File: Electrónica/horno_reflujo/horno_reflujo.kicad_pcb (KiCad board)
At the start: 2 copper layers, 100 x 80 mm, 46 parts, among them J1 LevelShifter, J10 ssr1, J11 ssr2, J12 encoder, J13 Max6675_modulo2, J14 Max6675_modulo3, J15 Max6675_modulo4, J2 LevelShifter, J3 Display Oled I2C, J4 Max6675_modulo, J5 ESP01, J6 Alimentación y zc, J7 Relevador a ventilador, J8 resistencia, K1 SANYOU_SRD_Form_C, Q1 2N2222A-TO92, U1 LD1117S33TR_SOT223, U2 74LS14

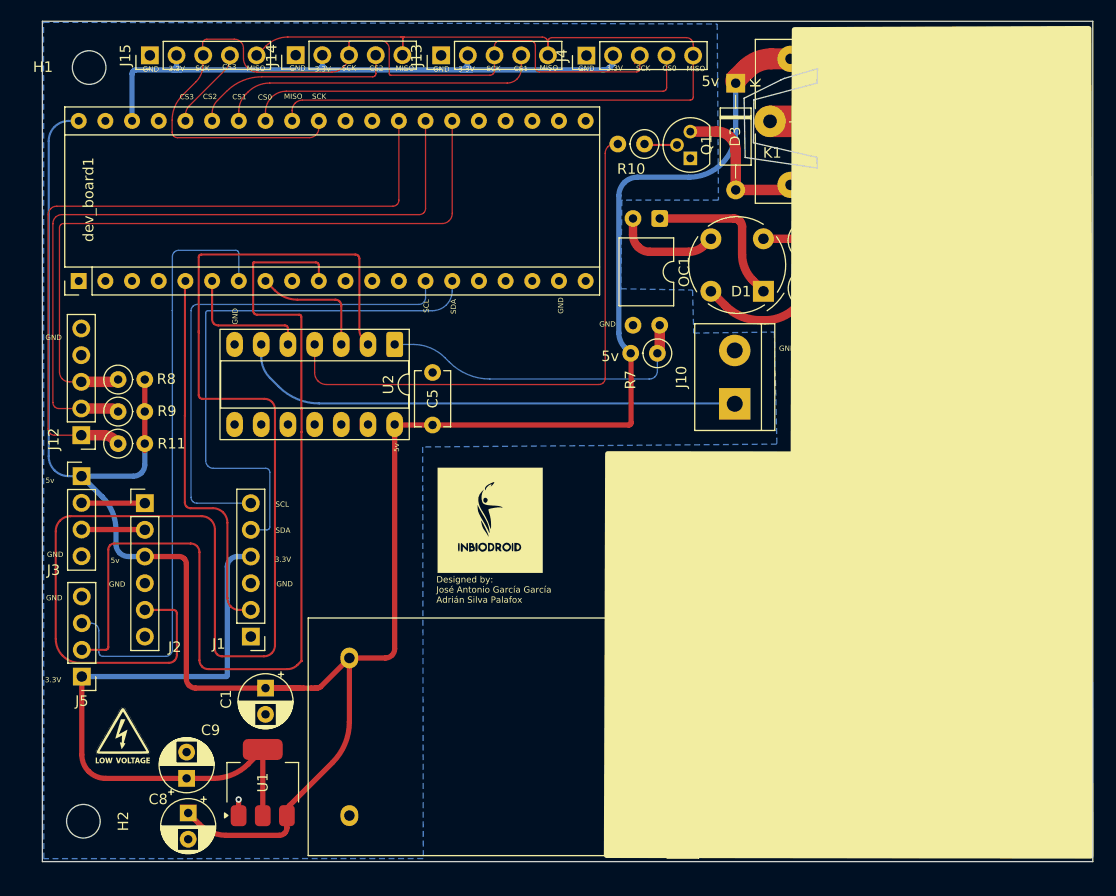
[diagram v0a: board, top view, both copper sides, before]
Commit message: mounting holes update
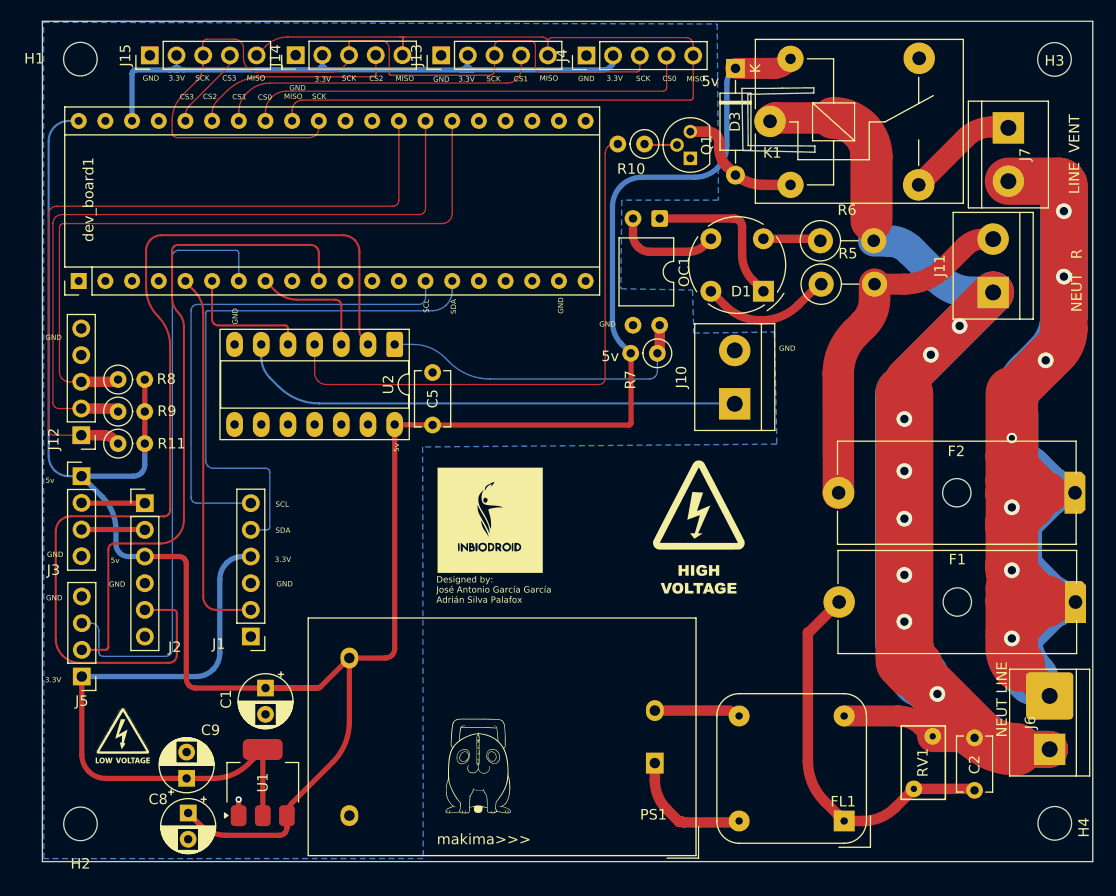
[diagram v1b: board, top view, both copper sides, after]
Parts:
- removed J8: resistencia, Connector_PinHeader_2.54mm:PinHeader_1x01_P2.54mm_Vertical
- added G***: LOGO, LOGO, F.Cu at (76.5, 97.2)
- moved D3 1.41 mm to (101.0, 30.8)
- moved R5 1.28 mm to (109.1, 51.3)
- moved H1 1.16 mm to (38.6, 29.9)
- moved R6 1.15 mm to (109.1, 47.2)
- moved H3 0.55 mm to (131.3, 29.9)
- moved H2 0.37 mm to (38.6, 102.7), turned to 180 degrees
- moved H4 0.20 mm to (131.4, 102.7)
- moved J11 0.11 mm to (125.5, 52.1)
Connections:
- F2 pad 2: Net-(J8-Pin_1) -> Net-(J11-Pin_2)
- J11 pad 2: unconnected-(J11-Pin_2-Pad2) -> Net-(J11-Pin_2)
- R5 pad 2: Net-(J8-Pin_1) -> Net-(J11-Pin_2)
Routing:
- net zero: track 133.3 -> 99.1 mm
- net Net-(J11-Pin_2): track 0.00 -> 33.6 mm
- net /Rx_mcu_esp01: track 92.3 -> 64.0 mm
- net Net-(J8-Pin_1): track 27.5 -> 0.00 mm
- net NEUT: track 176.7 -> 172.0 mm
- net Net-(D1-1): track 4.32 -> 6.62 mm
- net +3.3Vmc: track 58.5 -> 60.7 mm
- net +5V: track 224.9 -> 227.0 mm
- net Net-(D3-A): track 14.5 -> 12.7 mm
- net +3.3V: track 62.1 -> 60.8 mm
- net LINE: track 178.5 -> 177.4 mm
- net Net-(D1-2): track 11.6 -> 12.6 mm
- net SPI1_SCK: track 82.6 -> 82.0 mm
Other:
- outline, holes or cut-outs redrawn
- board text added: "NEUT R"
- board text added: "makima>>>"
- board text removed: "NEUT SSR"
- board text removed: "RESISTENCIA"

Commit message: actualizacion de placa
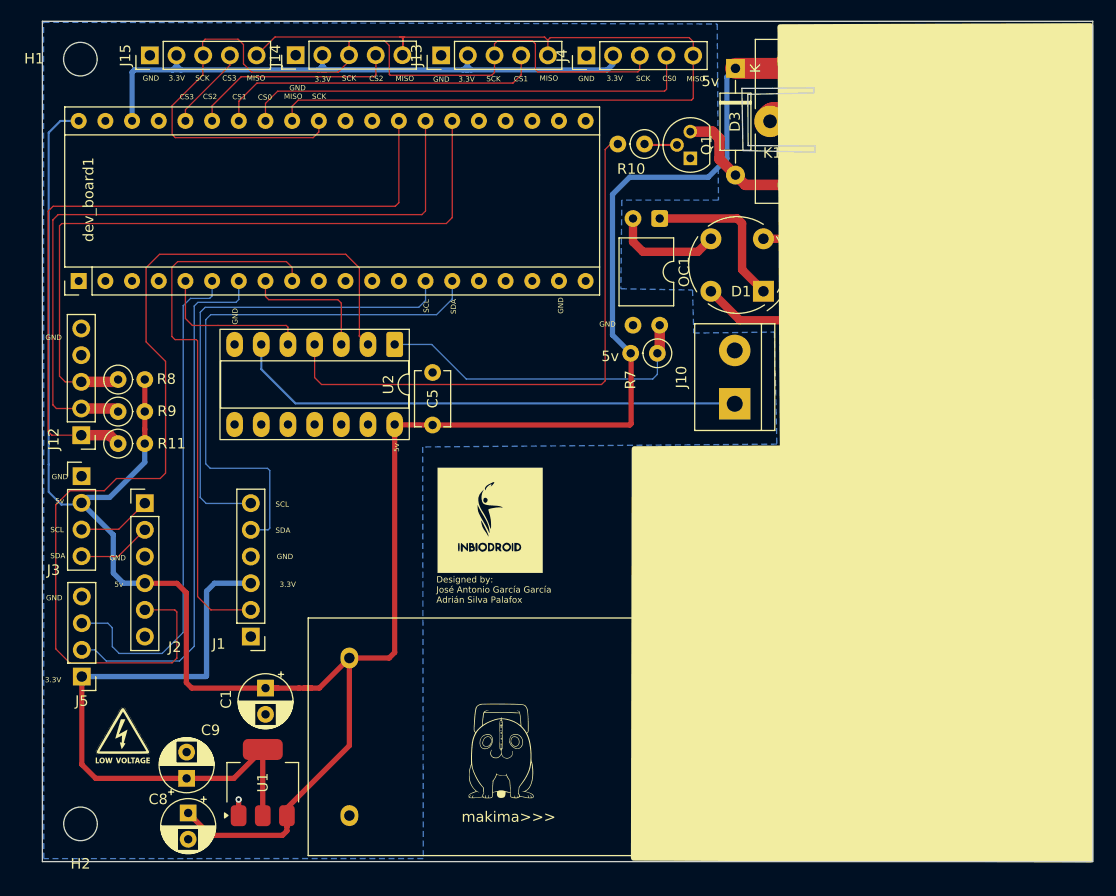
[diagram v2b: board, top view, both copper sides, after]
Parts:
- moved G*** 2.62 mm to (78.7, 95.8)
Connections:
- J1 pad 3: GND -> +3.3V
- J1 pad 4: +3.3V -> GND
- J2 pad 3: +5V -> GND
- J2 pad 4: GND -> +5V
- J3 pad 1: +5V -> GND
- J3 pad 2: Net-(J2-Pin_1) -> +5V
- J3 pad 3: Net-(J2-Pin_2) -> Net-(J2-Pin_1)
- J3 pad 4: GND -> Net-(J2-Pin_2)
- dev_board1 pad 10: /Rx_mcu_esp01 -> unconnected-(dev_board1-A15-Pad10)
- dev_board1 pad 5: /zc -> /fire
- dev_board1 pad 6: /fire -> /Tx_mcu_esp01
- dev_board1 pad 7: /Tx_mcu_esp01 -> /Rx_mcu_esp01
- dev_board1 pad 9: unconnected-(dev_board1-A12-Pad9) -> /zc
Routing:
- net /zc: track 36.6 -> 52.7 mm
- net /Rx_mcu_esp01: track 64.0 -> 50.4 mm
- net /Tx_mcu_esp01: track 59.0 -> 48.9 mm
- net zero: track 99.1 -> 94.5 mm
- net /fire: track 12.9 -> 15.9 mm
- net I2C1_SCL: track 48.6 -> 47.1 mm
- net +5V: track 227.0 -> 228.4 mm
- net +3.3V: track 60.8 -> 59.6 mm
- net Net-(J2-Pin_2): track 6.03 -> 7.13 mm
- net /fan: track 11.8 -> 12.9 mm
- net SPI1_SCK: track 82.0 -> 83.1 mm
- net Net-(J2-Pin_1): track 6.03 -> 7.06 mm
- net NEUT: track 172.0 -> 171.2 mm
- net Net-(J11-Pin_2): track 33.6 -> 34.4 mm
- net Net-(D3-A): track 12.7 -> 13.5 mm
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
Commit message: final check
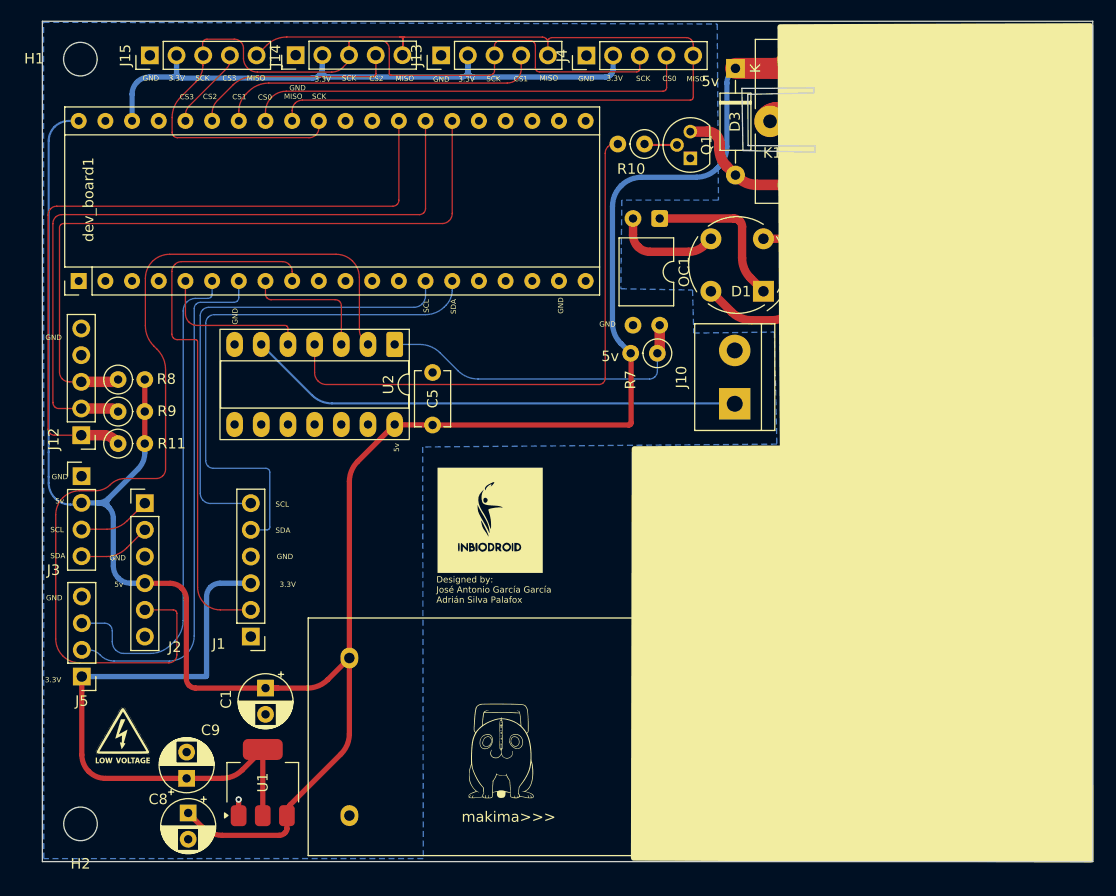
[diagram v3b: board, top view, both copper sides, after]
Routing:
- net NEUT: track 171.2 -> 161.2 mm
- net LINE: track 177.5 -> 170.9 mm
- net +5V: track 228.4 -> 225.0 mm
- net zero: track 94.5 -> 93.0 mm
- net Net-(J10-Pin_1): track 48.8 -> 47.3 mm
- net SPI1_SCK: track 83.1 -> 82.1 mm
- net Net-(D3-A): track 13.5 -> 12.7 mm
- net /Tx_mcu_esp01: track 48.9 -> 48.3 mm
- net /zc: track 52.7 -> 52.2 mm
- net Net-(J11-Pin_2): track 34.4 -> 33.9 mm
